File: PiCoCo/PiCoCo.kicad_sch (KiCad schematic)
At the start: 8 parts, among them IC1 74FST3257DR2G, IC2 74FST3257DR2G, J1 Conn_01x02_Pin, U1 Pico, U2 74HC244, U3 74HC244

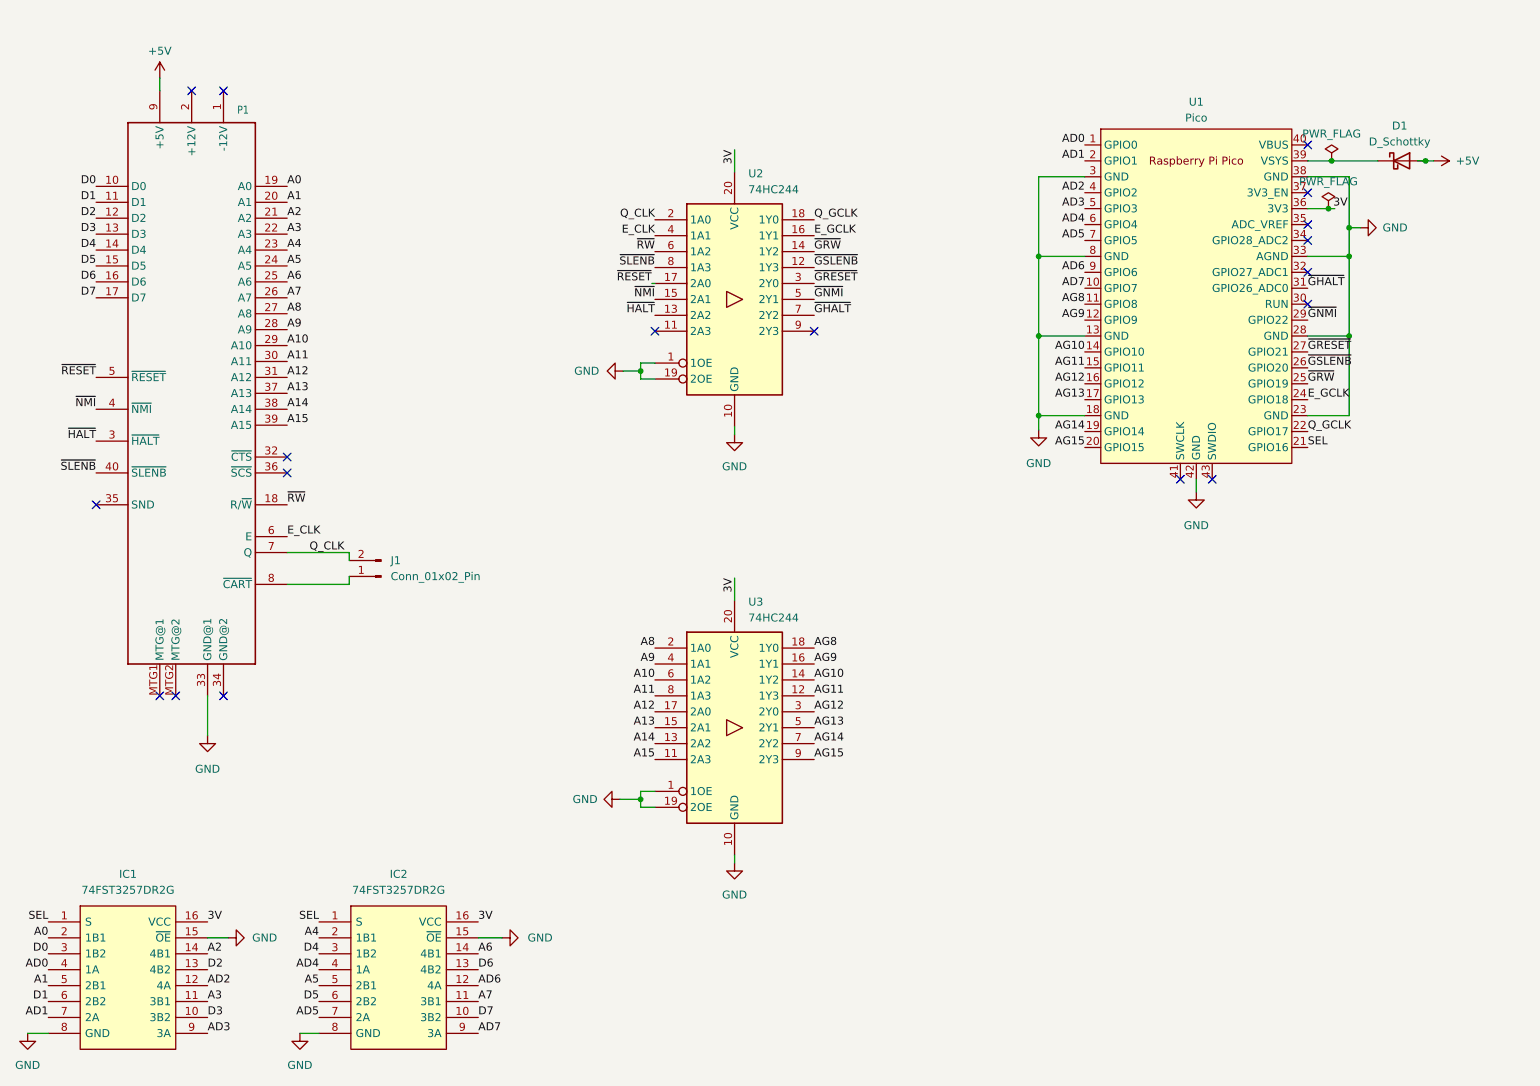
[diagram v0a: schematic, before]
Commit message: Updated initial PCB
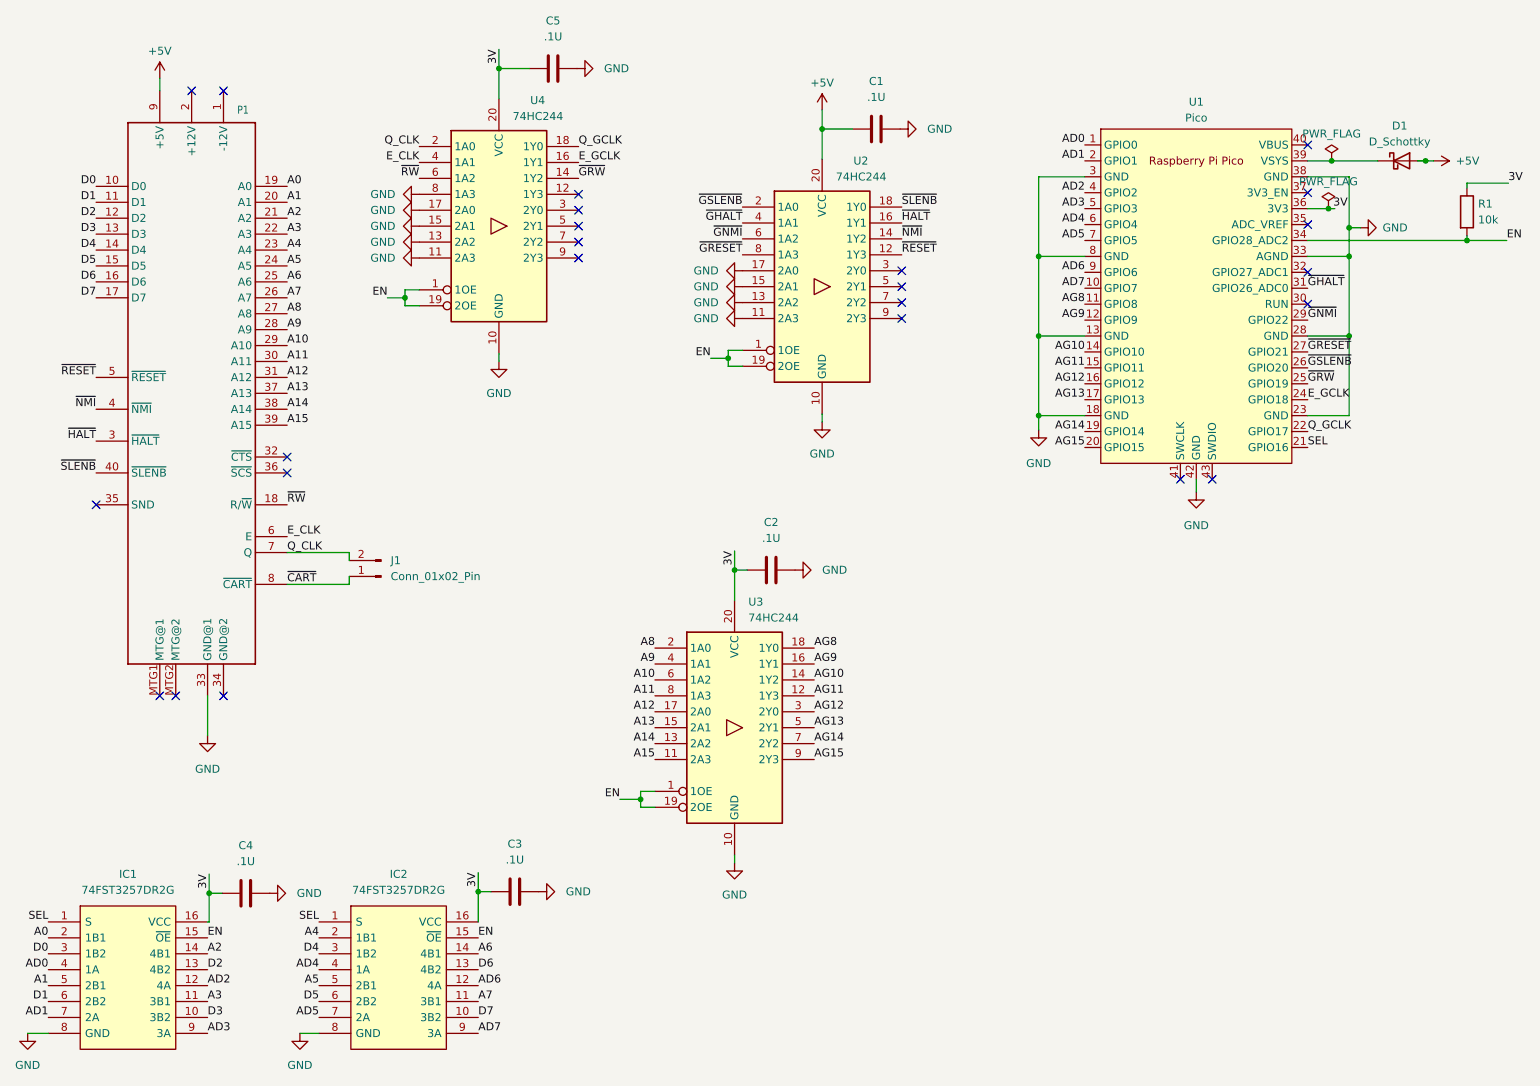
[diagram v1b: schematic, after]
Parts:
- added C1, C2, C3, C4, C5: .1U, Capacitor_SMD:C_0201_0603Metric_Pad0.64x0.40mm_HandSolder, symbol Device:C
- added R1: 10k, Resistor_SMD:R_0201_0603Metric_Pad0.64x0.40mm_HandSolder, symbol Device:R
- added U4: 74HC244, Package_SO:TSSOP-20_4.4x6.5mm_P0.65mm, symbol 74xx:74HC244
- IC1, IC2: footprint SOIC127P600X175-16N -> Package_SO:TSSOP-16_4.4x5mm_P0.65mm
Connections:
- net +5V: now also U2.20 (VCC), C1.2
- net 3V: now also C2.2, C3.2, C4.2, C5.2, R1.1, U4.20 (VCC); no longer U2.20 (VCC)
- net E_CLK: now also U4.4 (1A1); no longer U2.4 (1A1)
- net E_GCLK: now also U4.16 (1Y1); no longer U2.16 (1Y1)
- net GND: now also U2.11 (2A3), U2.13 (2A2), U2.15 (2A1), U2.17 (2A0), C1.1, C2.1, C3.1, C4.1, C5.1, U4.10 (GND), U4.11 (2A3), U4.13 (2A2), U4.15 (2A1), U4.17 (2A0), U4.8 (1A3); no longer IC1.15 (~{OE}), IC2.15 (~{OE}), U2.1 (1OE), U2.19 (2OE), U3.1 (1OE), U3.19 (2OE)
- net Q_CLK: now also U4.2 (1A0); no longer U2.2 (1A0)
- net Q_GCLK: now also U4.18 (1Y0); no longer U2.18 (1Y0)
- net ~{GHALT}: now also U2.4 (1A1); no longer U2.7 (2Y2)
- net ~{GNMI}: now also U2.6 (1A2); no longer U2.5 (2Y1)
- net ~{GRESET}: now also U2.8 (1A3); no longer U2.3 (2Y0)
- net ~{GRW}: now also U4.14 (1Y2); no longer U2.14 (1Y2)
- net ~{GSLENB}: now also U2.2 (1A0); no longer U2.12 (1Y3)
- net ~{HALT}: now also U2.16 (1Y1); no longer U2.13 (2A2)
- net ~{NMI}: now also U2.14 (1Y2); no longer U2.15 (2A1)
- net ~{RESET}: now also U2.12 (1Y3); no longer U2.17 (2A0)
- net ~{RW}: now also U4.6 (1A2); no longer U2.6 (1A2)
- net ~{SLENB}: now also U2.18 (1Y0); no longer U2.8 (1A3)
- net ~{CART}: now reaches J1.1 (Pin_1), P1.8 (~{CART})
- net EN: now reaches U1.34 (GPIO28_ADC2)
- net EN: now also IC1.15 (~{OE}), IC2.15 (~{OE}), U2.1 (1OE), U2.19 (2OE), U3.1 (1OE), U3.19 (2OE), R1.2, U4.1 (1OE), U4.19 (2OE)
- no-connect marks 18 -> 24
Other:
- moved on the sheet: U2
